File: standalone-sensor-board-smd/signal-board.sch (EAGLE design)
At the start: 32 parts, among them Q1 QRE1113, Q2 QRE1113, Q3 QRE1113, Q4 QRE1113, Q5 QRE1113, Q6 QRE1113, Q7 QRE1113, U1 CD4051BE

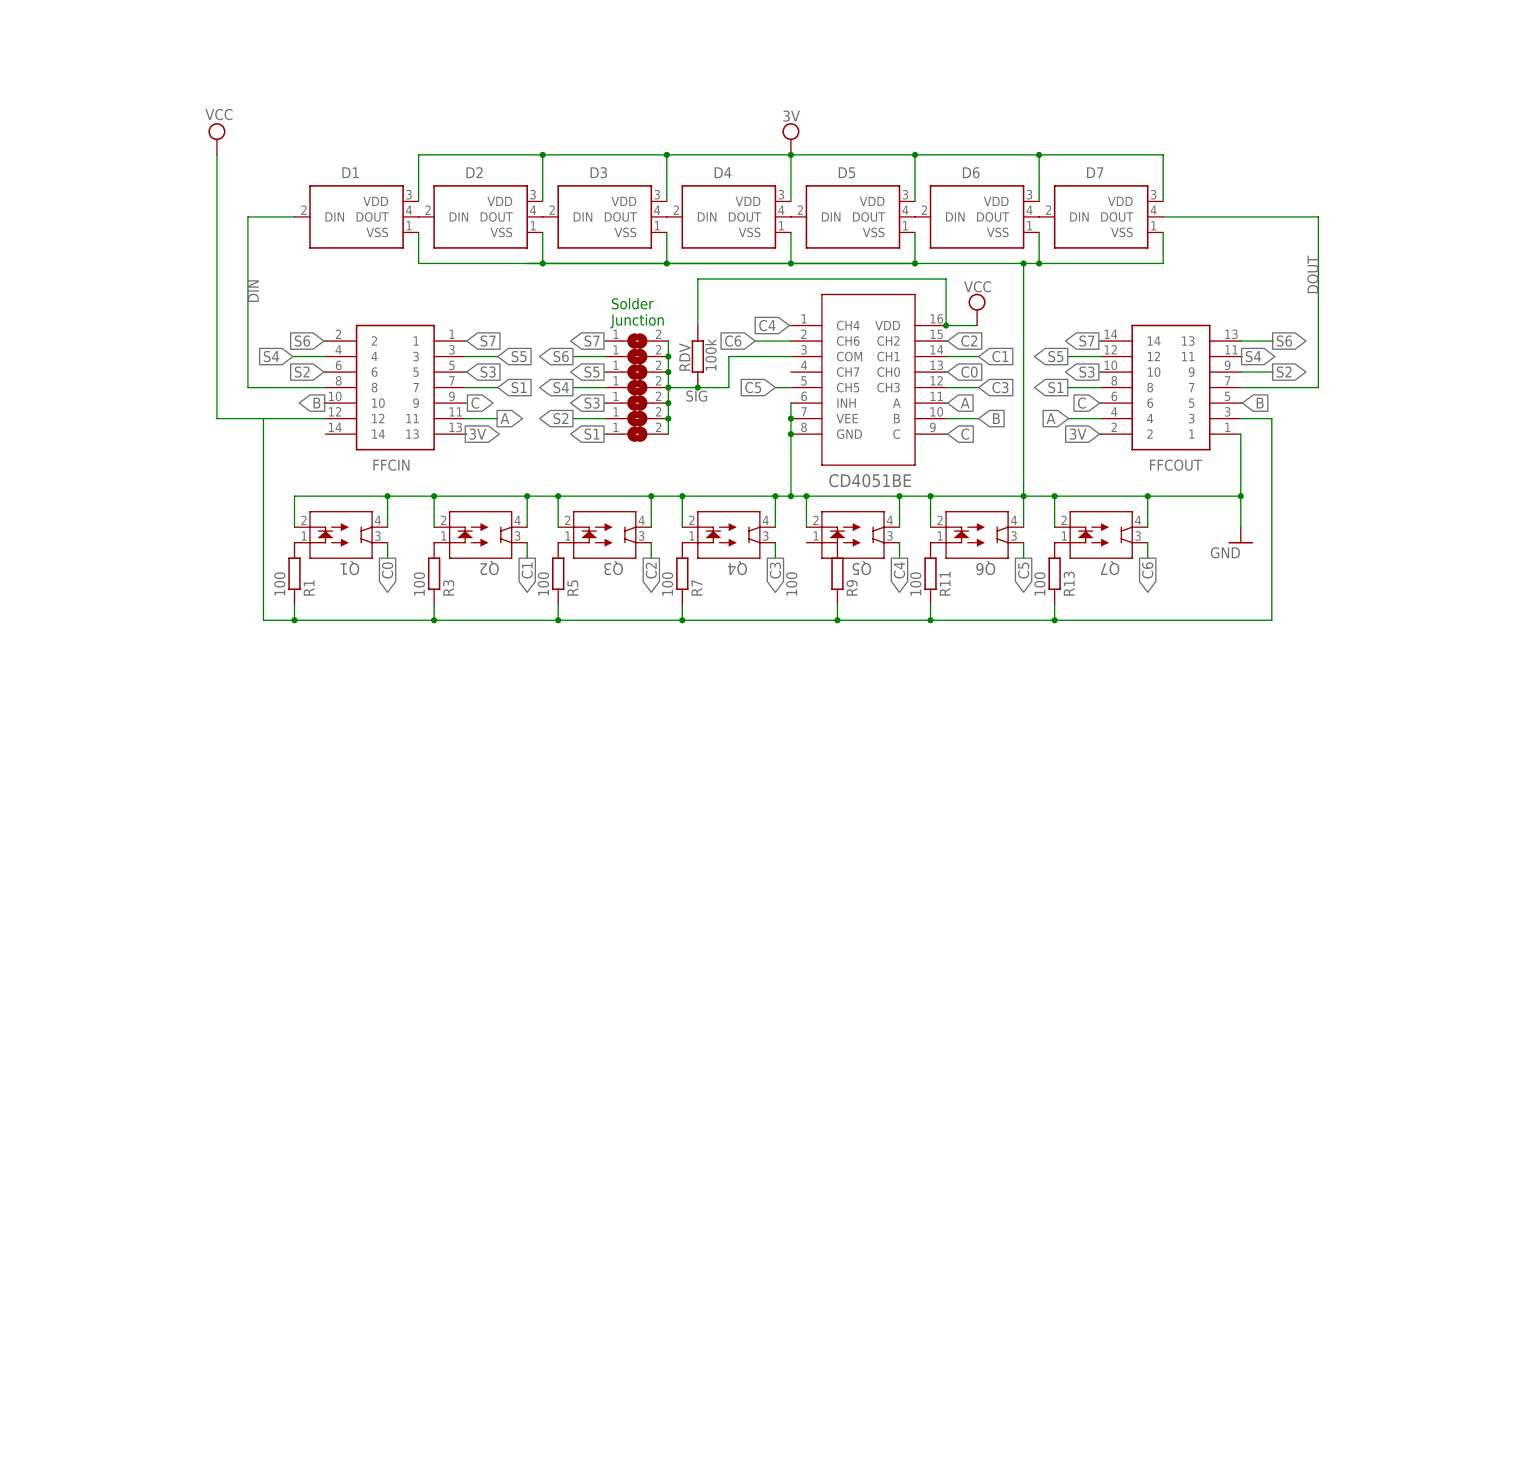
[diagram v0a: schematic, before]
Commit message: add smd boards from standalone
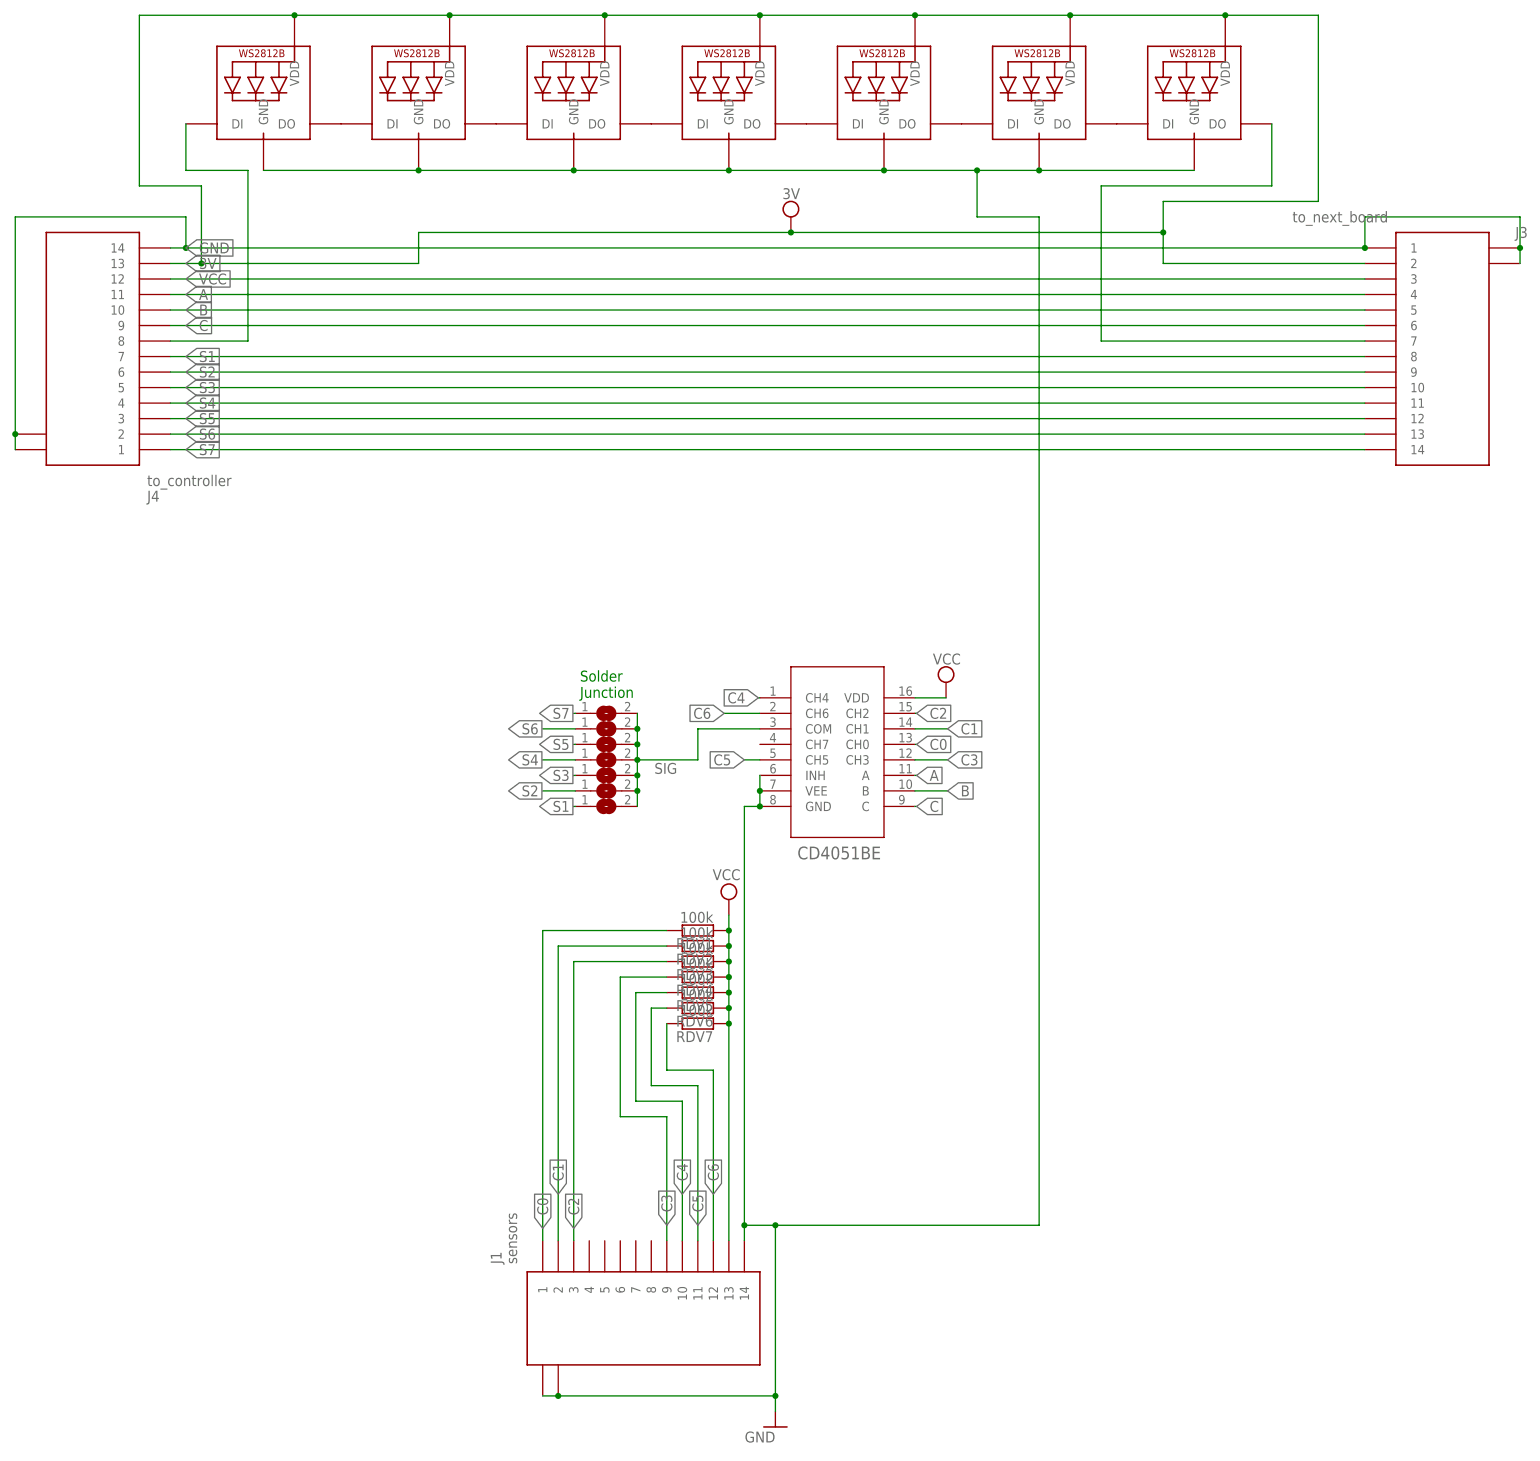
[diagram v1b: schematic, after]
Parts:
- removed D1, D2, D3, D4, D5, D6, D7: 1655, 1655:1655
- removed FFCIN, FFCOUT: 52806-1410, 52806-1410:52806-1410
- removed Q1, Q2, Q3, Q4, Q5, Q6, Q7: QRE1113, qre1113:QRE1113
- removed R1, R11, R13, R3, R5, R7, R9: 100, rcl:R-EU_0207/10
- removed RDV: 100k, rcl:R-EU_0207/10
- added J1: sensors, 686114148922:686114148922
- added J3: to_next_board, 686114148922:686114148922
- added J4: to_controller, 686114148922:686114148922
- added LED1, LED2, LED3, LED4, LED5, LED6, LED7: WS2812B3535, adafruit:WS2812B3535
- added RDV1, RDV2, RDV3, RDV4, RDV5, RDV6, RDV7: 100k, rcl:R-EU_0207/10
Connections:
- removed net N$11: Q6.1, R11.2
- removed net N$13: Q7.1, R13.2
- removed net N$15: D6.DOUT, D7.DIN
- removed net N$16: D1.DOUT, D2.DIN
- removed net N$17: D2.DOUT, D3.DIN
- removed net N$18: D3.DOUT, D4.DIN
- removed net N$19: D4.DOUT, D5.DIN
- removed net N$20: D5.DOUT, D6.DIN
- removed net N$7: Q4.1, R7.2
- new net N$4: LED4.DO, LED5.DI
- new net N$6: LED6.DO, LED7.DI
- net 3V: now also J3.2, J4.13, LED1.VDD, LED2.VDD, LED3.VDD, LED4.VDD, LED5.VDD, LED6.VDD, LED7.VDD; no longer D1.VDD, D2.VDD, D3.VDD, D4.VDD, D5.VDD, D6.VDD, D7.VDD, FFCIN.13, FFCOUT.2
- net A: now also J3.4, J4.11; no longer FFCIN.11, FFCOUT.4
- net B: now also J3.5, J4.10; no longer FFCIN.10, FFCOUT.5
- net C: now also J3.6, J4.9; no longer FFCIN.9, FFCOUT.6
- net C0: now also J1.1, RDV1.2; no longer Q1.3
- net C1: now also J1.2, RDV2.2; no longer Q2.3
- net C2: now also J1.3, RDV3.2; no longer Q3.3
- net C3: now also J1.9, RDV4.2; no longer Q4.3
- net C4: now also J1.10, RDV5.2; no longer Q5.3
- net C5: now also J1.11, RDV6.2; no longer Q6.3
- net C6: now also J1.12, RDV7.2; no longer Q7.3
- net DIN: now also J4.8, LED1.DI; no longer D1.DIN, FFCIN.8
- net DOUT: now also J3.7, LED7.DO; no longer D7.DOUT, FFCOUT.7
- net GND: now also J1.14, J1.MP1, J1.MP2, J3.1, J3.MP1, J3.MP2, J4.14, J4.MP1, J4.MP2, LED1.GND, LED2.GND, LED3.GND, LED4.GND, LED5.GND, LED6.GND, LED7.GND; no longer D1.VSS, D2.VSS, D3.VSS, D4.VSS, D5.VSS, D6.VSS, D7.VSS, FFCOUT.1, Q1.2, Q1.4, Q2.2, Q2.4, Q3.2, Q3.4, Q4.2, Q4.4, Q5.2, Q5.4, Q6.2, Q6.4, Q7.2, Q7.4
- net N$1: now also LED1.DO, LED2.DI; no longer Q1.1, R1.2
- net N$2: now also LED2.DO, LED3.DI; no longer FFCOUT.3, R1.1, R11.1, R13.1, R3.1, R5.1, R7.1, R9.1
- net N$3: now also LED3.DO, LED4.DI; no longer Q2.1, R3.2
- net N$5: now also LED5.DO, LED6.DI; no longer Q3.1, R5.2
- net S1: now also J3.8, J4.7; no longer FFCIN.7, FFCOUT.8
- net S2: now also J3.9, J4.6; no longer FFCIN.6, FFCOUT.9
- net S3: now also J3.10, J4.5; no longer FFCIN.5, FFCOUT.10
- net S4: now also J3.11, J4.4; no longer FFCIN.4, FFCOUT.11
- net S5: now also J3.12, J4.3; no longer FFCIN.3, FFCOUT.12
- net S6: now also J3.13, J4.2; no longer FFCIN.2, FFCOUT.13
- net S7: now also J3.14, J4.1; no longer FFCIN.1, FFCOUT.14
- net SIG: no longer RDV.1
- net VCC: now also J1.13, J3.3, J4.12, RDV1.1, RDV2.1, RDV3.1, RDV4.1, RDV5.1, RDV6.1, RDV7.1; no longer FFCIN.12, RDV.2
